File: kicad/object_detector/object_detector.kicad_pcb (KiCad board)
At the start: 2 copper layers, 82.2 x 69.4 mm, 27 parts, among them U1 LM386, U2 ESP32_DevKitC, U3 NCP1117-5.0_SOT223

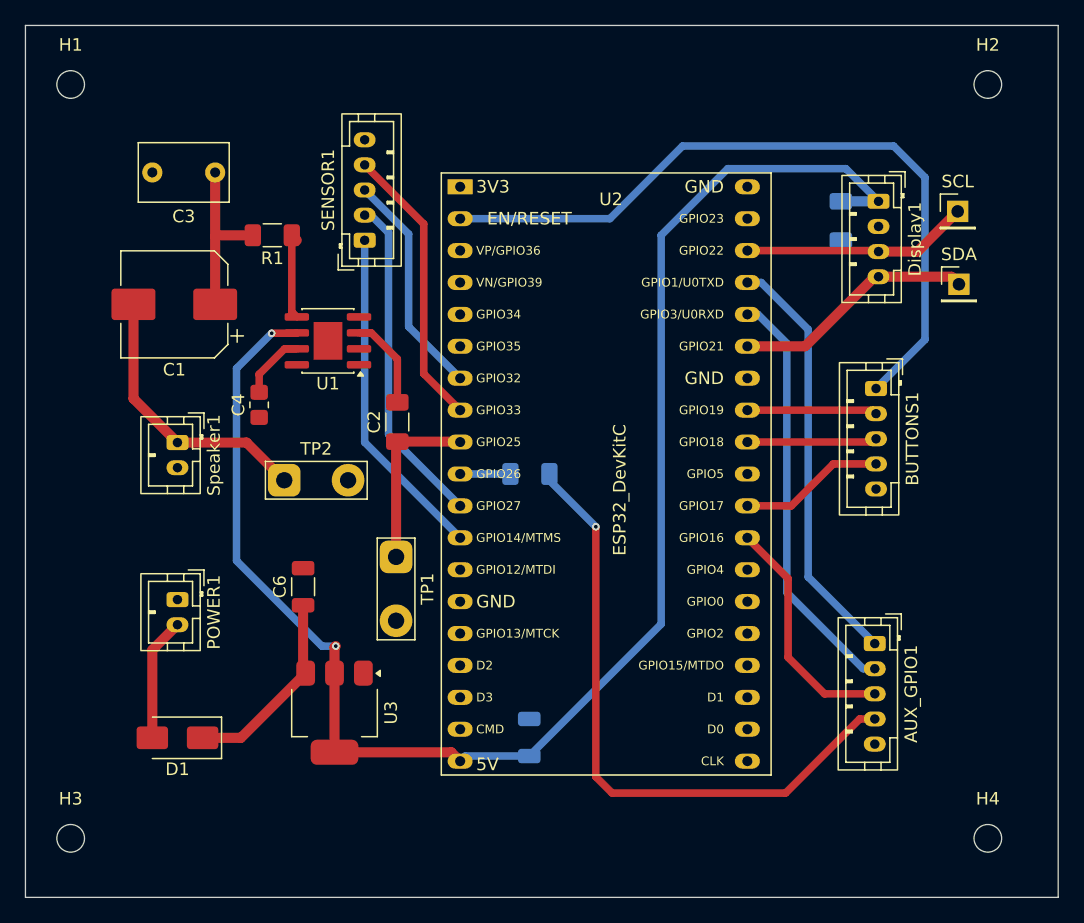
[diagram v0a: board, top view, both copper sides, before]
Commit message: PCB edits, MC code edits
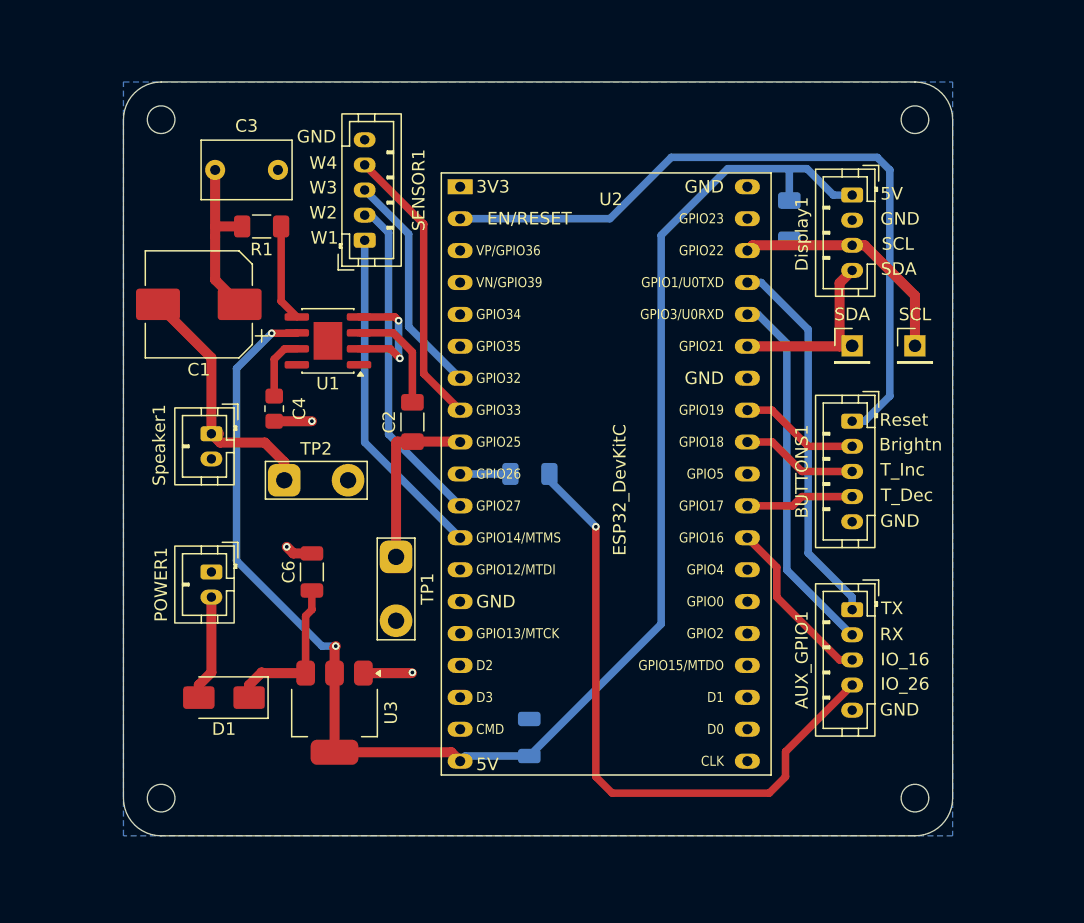
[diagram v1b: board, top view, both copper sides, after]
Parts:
- added G***: LOGO, Graphics:Abbey image, B.Cu at (153.7, 79.6)
- moved SCL 11.2 mm to (174.0, 85.0)
- moved SDA 9.81 mm to (169.0, 85.0)
- moved H3 7.88 mm to (114.0, 121.0)
- moved H1 7.73 mm to (114.0, 67.0)
- moved H4 6.62 mm to (174.0, 121.0)
- moved H2 6.44 mm to (174.0, 67.0)
- moved D1 4.89 mm to (119.0, 113.0)
- moved C5 4.10 mm to (164.0, 75.0)
- moved POWER1 3.48 mm to (118.0, 103.0)
- moved AUX_GPIO1 3.24 mm to (169.0, 106.0)
- moved BUTTONS1 3.22 mm to (169.0, 91.0)
- moved Speaker1 2.79 mm to (118.0, 92.0)
- moved Display1 2.16 mm to (169.0, 73.0)
- moved C1 1.95 mm to (117.0, 81.7)
- moved C6 1.37 mm to (126.0, 103.0)
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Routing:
- net GND: track 0.00 -> 19.0 mm, vias 0 -> 5
- net GPIO_16: track 19.0 -> 13.8 mm
- net SDA: track 19.4 -> 14.8 mm
- net RX: track 33.4 -> 29.5 mm
- net TX: track 33.6 -> 30.1 mm
- net TIME_DEC: track 11.6 -> 8.65 mm
- net 5V: track 126.1 -> 123.1 mm
- net Net-(D1-K): track 15.8 -> 13.1 mm
- net Net-(U1-+): track 7.36 -> 8.88 mm
- net Net-(D1-A): track 9.83 -> 8.41 mm
- net Net-(Speaker1-Pin_1): track 22.2 -> 20.8 mm
- net SCL: track 18.1 -> 19.2 mm
- net TIME_INC: track 10.3 -> 9.31 mm
- net BRIGHTNESS: track 10.4 -> 9.53 mm
- added copper zone on B.Cu, net GND
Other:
- board size 82.2 x 69.4 mm -> 66 x 60 mm
- rule pad_to_mask_clearance: 0 -> 0.0508
- board text added: "5V"
- board text added: "Brightn"
- board text added: "GND"
- board text added: "IO_16"
- board text added: "IO_26"
- board text added: "Nicholas Gerbavac John Ramus Arthur Roth"
- board text added: "OBJECT DETECTOR ECE342"
- board text added: "RX"
- board text added: "Reset"
- board text added: "SCL"
- board text added: "SDA"
- board text added: "TX"
- board text added: "T_Dec"
- board text added: "T_Inc"
- board text added: "W1"
- board text added: "W2"
- board text added: "W3"
- board text added: "W4"
